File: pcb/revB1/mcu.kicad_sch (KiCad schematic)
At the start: 38 parts, among them J4 Micro_SD_Card, J5 Micro_SD_Card, U5 APS6404L-3SQR, U6 APS6404L-3SQR, U7 MKL02Z32VFG4, U8 GD25Q64ESIGR, U9 MIMXRT1062DVJ6B, Y1 24MHz, Y2 32768

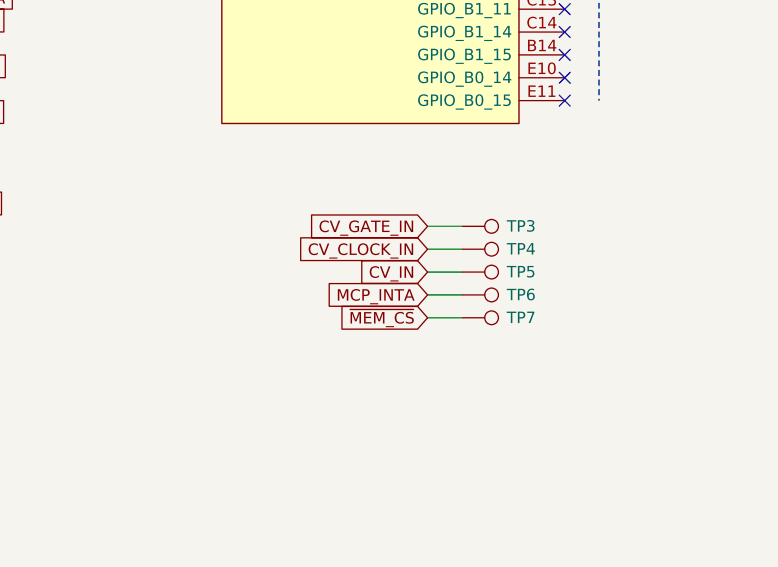
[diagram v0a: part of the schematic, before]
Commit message: Updated revB1
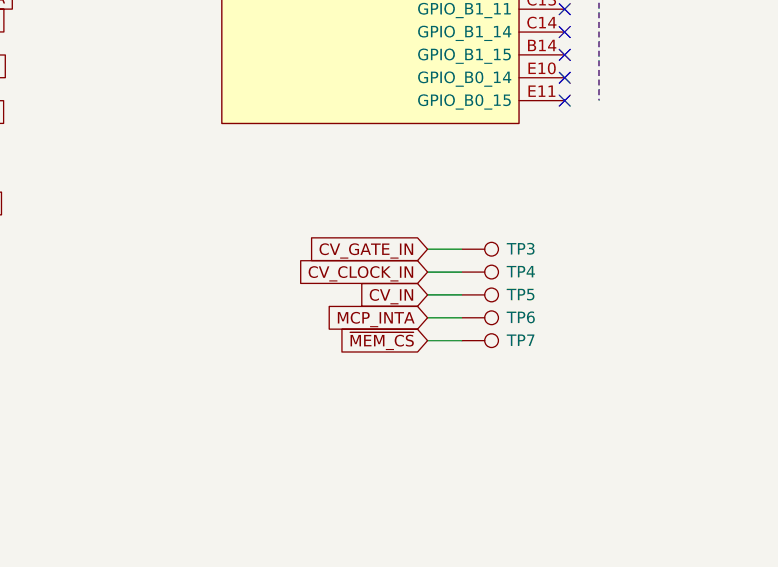
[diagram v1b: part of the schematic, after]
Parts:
- U9: footprint footprints:BGA196C80P14X14_1200X1200X152 -> MIMXRT1062DVJ6B:BGA196C80P14X14_1200X1200X152
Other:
- moved on the sheet: TP3, TP4, TP5, TP6, TP7
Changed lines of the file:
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@@
 	(wire
 		(pts
-			(xy 248.92 147.32) (xy 245.11 147.32)
+			(xy 248.92 149.86) (xy 245.11 149.86)
 		)
 		(stroke
@@
 	(wire
 		(pts
-			(xy 248.92 154.94) (xy 245.11 154.94)
+			(xy 248.92 157.48) (xy 245.11 157.48)
 		)
 		(stroke
@@
 	(wire
 		(pts
-			(xy 248.92 152.4) (xy 245.11 152.4)
+			(xy 248.92 154.94) (xy 245.11 154.94)
 		)
 		(stroke
@@
 	(wire
 		(pts
-			(xy 248.92 149.86) (xy 245.11 149.86)
+			(xy 248.92 152.4) (xy 245.11 152.4)
 		)
 		(stroke
@@
 	(wire
 		(pts
-			(xy 248.92 157.48) (xy 245.11 157.48)
+			(xy 248.92 160.02) (xy 245.11 160.02)
 		)
 		(stroke
@@
 	(global_label "CV_CLOCK_IN"
 		(shape input)
-		(at 245.11 149.86 180)
+		(at 245.11 152.4 180)
 		(fields_autoplaced yes)
 		(effects
@@
 		)
 		(property "Intersheetrefs" "${INTERSHEET_REFS}"
-			(at 229.7271 149.86 0)
+			(at 229.7271 152.4 0)
 			(hide yes)
 			(show_name no)
@@
 	(global_label "MCP_INTA"
 		(shape input)
-		(at 245.11 154.94 180)
+		(at 245.11 157.48 180)
 		(fields_autoplaced yes)
 		(effects
@@
 		)
 		(property "Intersheetrefs" "${INTERSHEET_REFS}"
-			(at 233.1743 154.94 0)
+			(at 233.1743 157.48 0)
 			(hide yes)
 			(show_name no)
@@
 	(global_label "CV_GATE_IN"
 		(shape input)
-		(at 245.11 147.32 180)
+		(at 245.11 149.86 180)
 		(fields_autoplaced yes)
 		(effects
@@
 		)
 		(property "Intersheetrefs" "${INTERSHEET_REFS}"
-			(at 231.4205 147.32 0)
+			(at 231.4205 149.86 0)
 			(hide yes)
 			(show_name no)
@@
 	(global_label "~{MEM_CS}"
 		(shape input)
-		(at 245.11 157.48 180)
+		(at 245.11 160.02 180)
 		(fields_autoplaced yes)
 		(effects
@@
 		)
 		(property "Intersheetrefs" "${INTERSHEET_REFS}"
-			(at 234.6259 157.48 0)
+			(at 234.6259 160.02 0)
 			(hide yes)
 			(show_name no)
@@
 	(global_label "CV_IN"
 		(shape input)
-		(at 245.11 152.4 180)
+		(at 245.11 154.94 180)
 		(fields_autoplaced yes)
 		(effects
@@
 		)
 		(property "Intersheetrefs" "${INTERSHEET_REFS}"
-			(at 236.8633 152.4 0)
+			(at 236.8633 154.94 0)
 			(hide yes)
 			(show_name no)
@@
 			)
 		)
-		(property "Footprint" "footprints:BGA196C80P14X14_1200X1200X152"
+		(property "Footprint" "MIMXRT1062DVJ6B:BGA196C80P14X14_1200X1200X152"
 			(at 145.542 149.352 0)
 			(hide yes)
@@
 	(symbol
 		(lib_id "Connector:TestPoint")
-		(at 248.92 149.86 270)
+		(at 248.92 152.4 270)
 		(unit 1)
 		(body_style 1)
@@
 		(dnp no)
 		(property "Reference" "TP4"
-			(at 255.524 149.86 90)
+			(at 255.524 152.4 90)
 			(show_name no)
 			(do_not_autoplace no)
@@
 		)
 		(property "Value" "CV CLOCK IN"
-			(at 252.222 152.4 90)
+			(at 252.222 154.94 90)
 			(hide yes)
 			(show_name no)
@@
 		)
 		(property "Footprint" "TestPoint:TestPoint_Pad_2.0x2.0mm"
-			(at 248.92 154.94 0)
+			(at 248.92 157.48 0)
 			(hide yes)
 			(show_name no)
@@
 		)
 		(property "Datasheet" ""
-			(at 248.92 154.94 0)
+			(at 248.92 157.48 0)
 			(hide yes)
 			(show_name no)
@@
 		)
 		(property "Description" "test point"
-			(at 248.92 149.86 0)
+			(at 248.92 152.4 0)
 			(hide yes)
 			(show_name no)
@@
 		)
 		(property "HighlightPins" "1"
-			(at 248.92 149.86 90)
+			(at 248.92 152.4 90)
 			(hide yes)
 			(show_name no)
@@
 	(symbol
 		(lib_id "Connector:TestPoint")
-		(at 248.92 154.94 270)
+		(at 248.92 157.48 270)
 		(unit 1)
 		(body_style 1)
@@
 		(dnp no)
 		(property "Reference" "TP6"
-			(at 255.524 154.94 90)
+			(at 255.524 157.48 90)
 			(show_name no)
 			(do_not_autoplace no)
@@
 		)
 		(property "Value" "MCP INTA"
-			(at 252.222 157.48 90)
+			(at 252.222 160.02 90)
 			(hide yes)
 			(show_name no)
@@
 		)
 		(property "Footprint" "TestPoint:TestPoint_Pad_2.0x2.0mm"
-			(at 248.92 160.02 0)
+			(at 248.92 162.56 0)
 			(hide yes)
 			(show_name no)
@@
 		)
 		(property "Datasheet" ""
-			(at 248.92 160.02 0)
+			(at 248.92 162.56 0)
 			(hide yes)
 			(show_name no)
@@
 		)
 		(property "Description" "test point"
-			(at 248.92 154.94 0)
+			(at 248.92 157.48 0)
 			(hide yes)
 			(show_name no)
@@
 		)
 		(property "HighlightPins" "1"
-			(at 248.92 154.94 90)
+			(at 248.92 157.48 90)
 			(hide yes)
 			(show_name no)
@@
 	(symbol
 		(lib_id "Connector:TestPoint")
-		(at 248.92 152.4 270)
+		(at 248.92 154.94 270)
 		(unit 1)
 		(body_style 1)
@@
 		(dnp no)
 		(property "Reference" "TP5"
-			(at 255.524 152.4 90)
+			(at 255.524 154.94 90)
 			(show_name no)
 			(do_not_autoplace no)
@@
 		)
 		(property "Value" "CV IN"
-			(at 252.222 154.94 90)
+			(at 252.222 157.48 90)
 			(hide yes)
 			(show_name no)
@@
 		)
 		(property "Footprint" "TestPoint:TestPoint_Pad_2.0x2.0mm"
-			(at 248.92 157.48 0)
+			(at 248.92 160.02 0)
 			(hide yes)
 			(show_name no)
@@
 		)
 		(property "Datasheet" ""
-			(at 248.92 157.48 0)
+			(at 248.92 160.02 0)
 			(hide yes)
 			(show_name no)
@@
 		)
 		(property "Description" "test point"
-			(at 248.92 152.4 0)
+			(at 248.92 154.94 0)
 			(hide yes)
 			(show_name no)
@@
 		)
 		(property "HighlightPins" "1"
-			(at 248.92 152.4 90)
+			(at 248.92 154.94 90)
 			(hide yes)
 			(show_name no)
@@
 			)
 		)
-		(property "Footprint" "footprints:BGA196C80P14X14_1200X1200X152"
+		(property "Footprint" "MIMXRT1062DVJ6B:BGA196C80P14X14_1200X1200X152"
 			(at 220.472 176.022 0)
 			(hide yes)
@@
 	(symbol
 		(lib_id "Connector:TestPoint")
-		(at 248.92 157.48 270)
+		(at 248.92 160.02 270)
 		(unit 1)
 		(body_style 1)
@@
 		(dnp no)
 		(property "Reference" "TP7"
-			(at 255.524 157.48 90)
+			(at 255.524 160.02 90)
 			(show_name no)
 			(do_not_autoplace no)
@@
 		)
 		(property "Value" "MEM CS"
-			(at 252.222 160.02 90)
+			(at 252.222 162.56 90)
 			(hide yes)
 			(show_name no)
@@
 		)
 		(property "Footprint" "TestPoint:TestPoint_Pad_2.0x2.0mm"
-			(at 248.92 162.56 0)
+			(at 248.92 165.1 0)
 			(hide yes)
 			(show_name no)
@@
 		)
 		(property "Datasheet" ""
-			(at 248.92 162.56 0)
+			(at 248.92 165.1 0)
 			(hide yes)
 			(show_name no)
@@
 		)
 		(property "Description" "test point"
-			(at 248.92 157.48 0)
+			(at 248.92 160.02 0)
 			(hide yes)
 			(show_name no)
@@
 		)
 		(property "HighlightPins" "1"
-			(at 248.92 157.48 90)
+			(at 248.92 160.02 90)
 			(hide yes)
 			(show_name no)
@@
 	(symbol
 		(lib_id "Connector:TestPoint")
-		(at 248.92 147.32 270)
+		(at 248.92 149.86 270)
 		(mirror x)
 		(unit 1)
@@
 		(dnp no)
 		(property "Reference" "TP3"
-			(at 255.524 147.32 90)
+			(at 255.524 149.86 90)
 			(show_name no)
 			(do_not_autoplace no)
@@
 		)
 		(property "Value" "CV GATE IN"
-			(at 252.222 144.78 90)
+			(at 252.222 147.32 90)
 			(hide yes)
 			(show_name no)
@@
 		)
 		(property "Footprint" "TestPoint:TestPoint_Pad_2.0x2.0mm"
-			(at 248.92 142.24 0)
+			(at 248.92 144.78 0)
 			(hide yes)
 			(show_name no)
@@
 		)
 		(property "Datasheet" ""
-			(at 248.92 142.24 0)
+			(at 248.92 144.78 0)
 			(hide yes)
 			(show_name no)
@@
 		)
 		(property "Description" "test point"
-			(at 248.92 147.32 0)
+			(at 248.92 149.86 0)
 			(hide yes)
 			(show_name no)
@@
 		)
 		(property "HighlightPins" "1"
-			(at 248.92 147.32 90)
+			(at 248.92 149.86 90)
 			(hide yes)
 			(show_name no)
